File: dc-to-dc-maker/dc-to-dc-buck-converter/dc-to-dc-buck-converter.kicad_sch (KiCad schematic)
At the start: 10 parts, among them IC1 EL7104CNZ, J1 1715721, J2 1715721, J3 1-826629-6, U1 IRF640NPBF

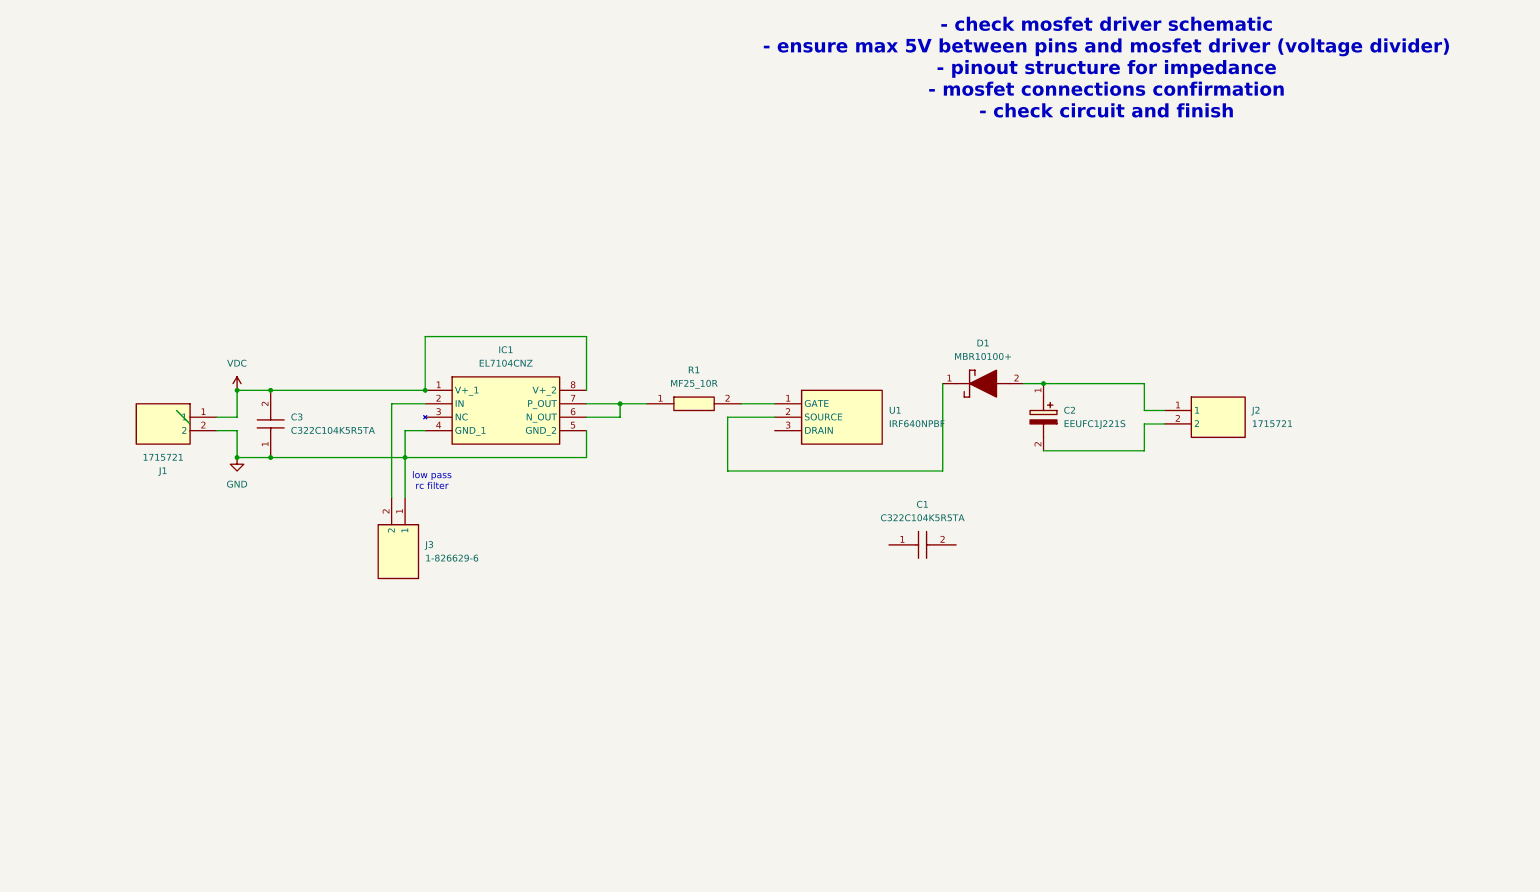
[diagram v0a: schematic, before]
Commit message: update
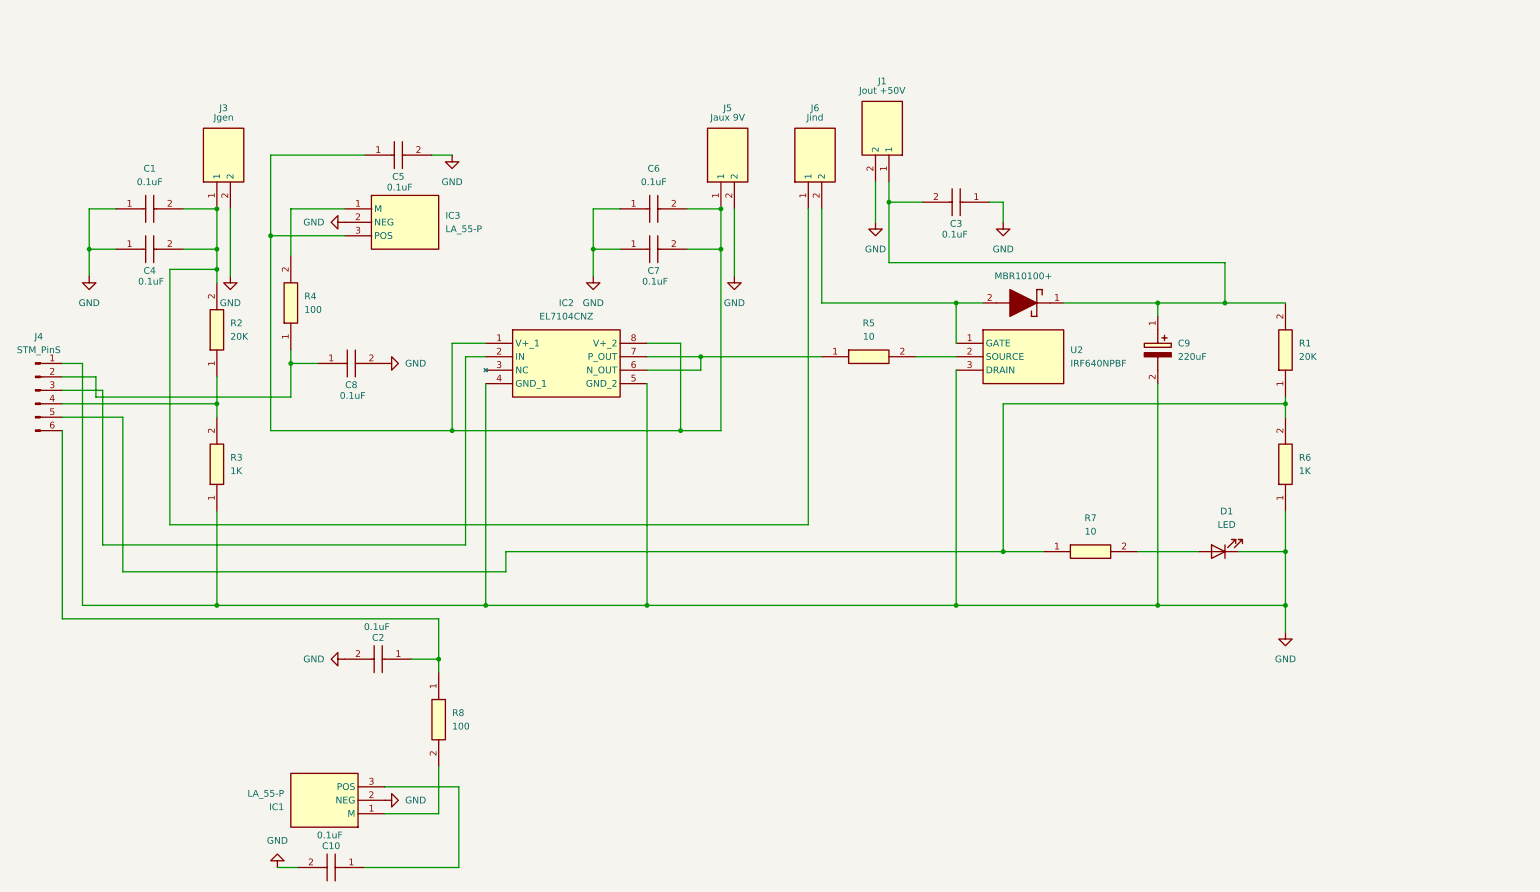
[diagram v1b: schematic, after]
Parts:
- removed C2: EEUFC1J221S, EEUFC1J221S(capacitor):CAPPRD500W65D1250H2200, symbol EEUFC1J221S(capacitor):EEUFC1J221S
- removed D1: MBR10100+, MBR10100+(diode):TO490P480X1000X2110-2P, symbol MBR10100+(diode):MBR10100+
- removed IC1: EL7104CNZ, EL7104CNZ(voltage regulator):DIP762W51P254L952H533Q8N, symbol EL7104CNZ(voltage regulator):EL7104CNZ
- removed J2: 1715721, 1715721(screw connector):1715721, symbol 1715721(screw connector):1715721
- removed J3: 1-826629-6, 1-826629-6(pins):HDRV16W63P0X254_1X16_4064X250X950P, symbol 1-826629-6(pins):1-826629-6
- removed R1: MF25_10R, RESAD1680W59L680D250, symbol MF25_10R(resistor):MF25_10R
- removed U1: IRF640NPBF, IRF640NPBF(mosfet):TO254P483X1016X1994-3P, symbol IRF640NPBF(mosfet):IRF640NPBF
- added C10, C2, C4, C5, C6, C7, C8: 0.1uF, C322C104K5R5TA(decoup capacitor):C322, symbol C322C104K5R5TA(decoup capacitor):C322C104K5R5TA
- added C9: 220uF, EEUFC1J221S(capacitor):CAPPRD500W65D1250H2200, symbol EEUFC1J221S(capacitor):EEUFC1J221S
- added D1: LED, symbol Device:LED
- added D2: MBR10100+, MBR10100+(diode):TO490P480X1000X2110-2P, symbol MBR10100+(diode):MBR10100+
- added IC1, IC3: LA_55-P, LA_55-P(current detector):LA55-P, symbol LA_55-P(current-sensor):LA_55-P
- added IC2: EL7104CNZ, EL7104CNZ(voltage regulator):DIP762W51P254L952H533Q8N, symbol EL7104CNZ(voltage regulator):EL7104CNZ
- added J3: Jgen, 1715721(screw connector):1715721, symbol 1715721(screw connector):1715721
- added J4: STM_PinS, Connector_Hirose:Hirose_DF63M-1P-3.96DSA_1x01_P3.96mm_Vertical, symbol Connector:Conn_01x06_Pin
- added J5: Jaux 9V, 1715721(screw connector):1715721, symbol 1715721(screw connector):1715721
- added J6: Jind, 1715721(screw connector):1715721, symbol 1715721(screw connector):1715721
- added R1, R2: 20K, MF25_20K(resistor):RESAD1680W59L680D250, symbol MF25_20K(resistor):MF25_20K
- added R3, R6: 1K, MF25_1K(resistor):RESAD1680W59L680D250, symbol MF25_1K(resistor):MF25_1K
- added R4, R8: 100, RESAD1680W59L680D250, symbol MF25_100R(resistor):MF25_100R
- added R5, R7: 10, RESAD1680W59L680D250, symbol MF25_10R(resistor):MF25_10R
- added U2: IRF640NPBF, IRF640NPBF(mosfet):TO254P483X1016X1994-3P, symbol IRF640NPBF(mosfet):IRF640NPBF
- C1, C3: value C322C104K5R5TA -> 0.1uF
- J1: value 1715721 -> Jout +50V
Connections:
- net GND: now also C1.1, C10.2, C2.2, C4.1, C5.2, C6.1, C7.1, C8.2, C9.2 (-), D1.1 (K), IC1.2 (NEG), IC2.4 (GND_1), IC2.5 (GND_2), IC3.2 (NEG), J3.2, J4.1 (Pin_1), J5.2, R3.1, R6.1, U2.3 (DRAIN)
- net at C1.2: now also C4.2, J3.1, J6.1, R2.2
- net VDC: no longer names the net of C3.2, J1.1
- net VDC: now also C9.1 (+), D2.1 (K), R1.2
- new net: C5.1, C6.2, C7.2, IC2.1 (V+_1), IC2.8 (V+_2), IC3.3 (POS), J5.1
- new net: C10.1, IC1.3 (POS)
- new net: J4.4 (Pin_4), R2.1, R3.2
- new net: IC2.6 (N_OUT), IC2.7 (P_OUT), R5.1
- new net: R5.2, U2.2 (SOURCE)
- new net: J4.5 (Pin_5), R1.1, R6.2, R7.1
- new net: D2.2 (A), J6.2, U2.1 (GATE)
- new net: IC1.1 (M), R8.2
- new net: C8.1, J4.2 (Pin_2), R4.1
- new net: C2.1, J4.6 (Pin_6), R8.1
- new net: IC3.1 (M), R4.2
- new net: IC2.2 (IN), J4.3 (Pin_3)
- new net: D1.2 (A), R7.2
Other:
- note removed: "- check mosfet driver schematic - ensure max 5V between pins and mosfet driver (voltage divider) - pinout structure for impedance - mosfet connections confirmation - check circuit and finish"
- note removed: "low pass rc filter"
- title: DC to DC Buck Boost Converter -> DC to DC Boost Converter
- moved on the sheet: C1
